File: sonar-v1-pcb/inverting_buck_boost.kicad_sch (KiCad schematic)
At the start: 1 part, among them U4 TPS54360DDAR

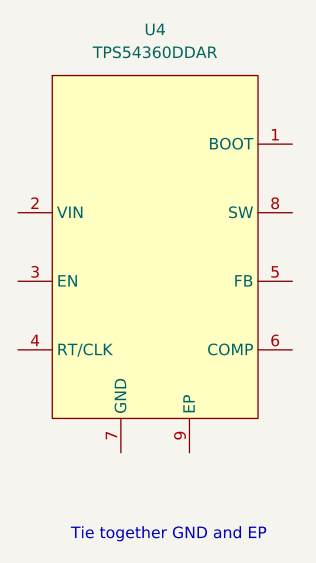
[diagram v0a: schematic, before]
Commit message: formatting lol
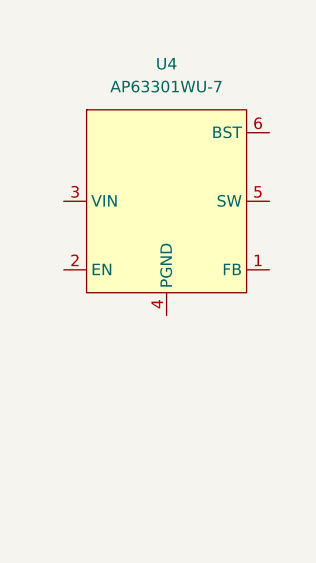
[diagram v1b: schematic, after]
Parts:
- removed U4: TPS54360DDAR, GS_SO:SOIC-8-1EP_3.9x4.9mm_P1.27mm_EP2.29x3mm, symbol GS_Switching_Regulators:TPS54360DDAR
- added U4: AP63301WU-7, Sonar:TSOT-23-6, symbol sonar_lib:AP63301WU-7
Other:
- note removed: "Tie together GND and EP"
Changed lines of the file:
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@@
 	(generator_version "9.0")
 	(paper "A4")
-	(text "Tie together GND and EP"
-		(exclude_from_sim no)
-		(at 148.844 131.064 0)
-		(effects
-			(font
-				(size 1.27 1.27)
-			)
-		)
-	)
 	(symbol
-		(lib_id "GS_Switching_Regulators:TPS54360DDAR")
-		(at 147.32 99.06 0)
+		(lib_id "sonar_lib:AP63301WU-7")
+		(at 148.59 93.98 0)
 		(unit 1)
 		(exclude_from_sim no)
@@
 		(fields_autoplaced yes)
 		(property "Reference" "U4"
-			(at 147.32 74.93 0)
+			(at 148.59 78.74 0)
 			(effects
 				(font
@@
 			)
 		)
-		(property "Value" "TPS54360DDAR"
-			(at 147.32 77.47 0)
+		(property "Value" "AP63301WU-7"
+			(at 148.59 81.28 0)
 			(effects
 				(font
@@
 			)
 		)
-		(property "Footprint" "GS_SO:SOIC-8-1EP_3.9x4.9mm_P1.27mm_EP2.29x3mm"
-			(at 147.32 66.04 0)
+		(property "Footprint" "Sonar:TSOT-23-6"
+			(at 148.59 63.5 0)
 			(effects
 				(font
@@
 			)
 		)
-		(property "Datasheet" "https://www.lcsc.com/datasheet/C44377.pdf"
-			(at 147.32 58.42 0)
+		(property "Datasheet" "https://www.lcsc.com/datasheet/C2158003.pdf"
+			(at 148.59 76.2 0)
 			(effects
 				(font
@@
 			)
 		)
-		(property "Description" "2.5MHz Adjustable Buck Converter, 4.5V-60V Input Voltage, 3.5A Max Current"
-			(at 147.32 68.58 0)
+		(property "Description" "500kHz Adjustable Buck Converter, 3A Max Current, 3.8V-32V Input Voltage"
+			(at 148.59 73.66 0)
 			(effects
 				(font
@@
 			)
 		)
-		(property "Manufacturer" "TI"
-			(at 147.32 73.66 0)
+		(property "Manufacturer" "DIODES"
+			(at 148.59 58.42 0)
 			(effects
 				(font
@@
 			)
 		)
-		(property "Mfr. Part #" "TPS54360DDAR"
-			(at 147.32 60.96 0)
+		(property "Mfr. Part #" "AP63301WU-7"
+			(at 148.59 60.96 0)
 			(effects
 				(font
@@
 			)
 		)
-		(property "LCSC ID" "C44377"
-			(at 147.32 63.5 0)
+		(property "LCSC ID" "C2158003"
+			(at 148.59 71.12 0)
 			(effects
 				(font
@@
 			)
 		)
-		(property "Package" "SOIC-8-EP"
-			(at 147.32 71.12 0)
+		(property "Package" "TSOT-23-6"
+			(at 148.59 68.58 0)
 			(effects
 				(font
@@
 			)
 		)
-		(pin "5"
+		(property "Spice Warning Override" "No SPICE model available"
+			(at 148.59 66.04 0)
+			(effects
+				(font
+					(size 1.27 1.27)
+				)
+				(hide yes)
+			)
 		)
 		(pin "4"
 		)
-		(pin "7"
+		(pin "2"
 		)
-		(pin "9"
+		(pin "1"
+		)
+		(pin "5"
+		)
+		(pin "6"
 		)
 		(pin "3"
 		)
-		(pin "8"
-		)
-		(pin "1"
-		)
-		(pin "2"
-		)
-		(pin "6"
-		)
 		(instances
